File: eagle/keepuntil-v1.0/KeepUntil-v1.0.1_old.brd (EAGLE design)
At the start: 37 x 45 mm, 18 parts, among them IC2 REG1117, J2 USBSMD, Q1 CSTCR6M00G53Z, T1 BC846, U1 ATMEGA328P-AU

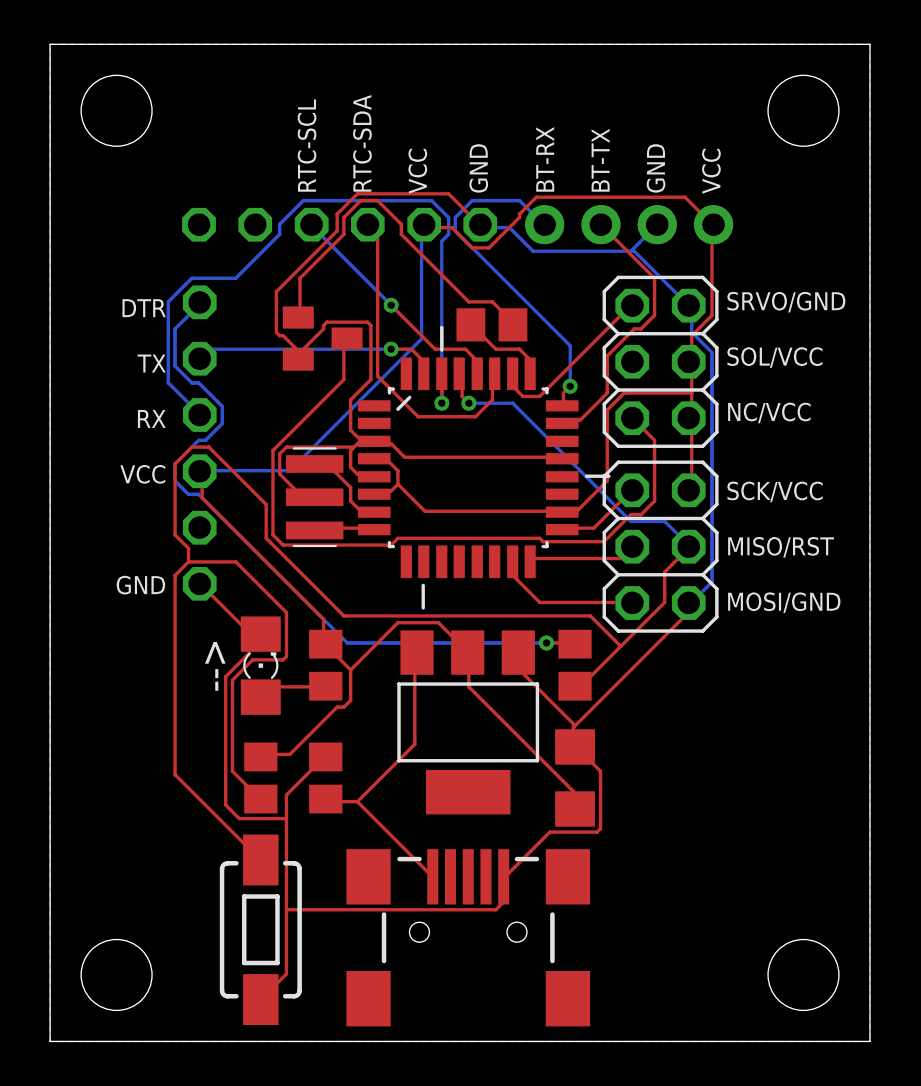
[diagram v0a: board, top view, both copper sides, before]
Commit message: new board layout
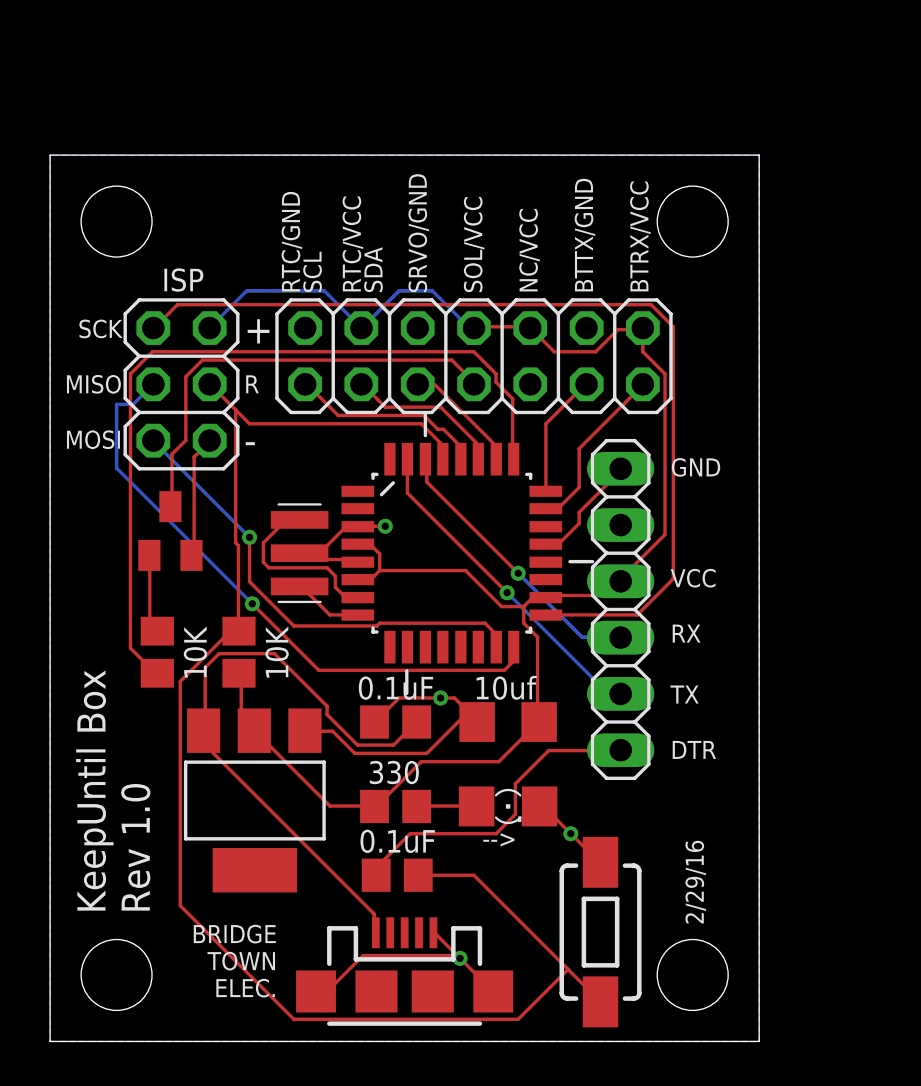
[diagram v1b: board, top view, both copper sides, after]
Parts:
- removed BLUETOOTH: 1X4-CLEANBIG, adafruit:1X04-CLEANBIG
- removed J2: USBSMD, SparkFun-Connectors:USB-MINIB
- removed LOCK-CTRL: (no value), pinhead:2X03
- removed RTC, RTC1: (no value), adafruit:1X06-CLEAN
- added J1: USB-MICROB, SparkFun-Connectors:USB-MICROB
- added JP1: (no value), pinhead:2X07
- added SERIAL: (no value), pinhead:1X06
- C1, C4: value .1uF -> 0.1uF
- moved ISP 22.8 mm to (5.93, 29.7)
- moved R2 21.1 mm to (4.84, 17.6), turned to 270 degrees
- moved S1 15.3 mm to (24.8, 4.93), turned to 270 degrees
- moved LED1 12.8 mm to (20.7, 10.6), turned to 0 degrees
- moved C1 12.4 mm to (15.7, 7.50), turned to 180 degrees
- moved T1 11.1 mm to (5.43, 23.0), turned to 0 degrees
- moved IC2 10.3 mm to (9.24, 10.9)
- moved R7 7.11 mm to (15.6, 10.6), turned to 180 degrees
- moved R1 5.76 mm to (8.53, 17.6), turned to 270 degrees
- moved C4 4.04 mm to (15.6, 14.4), turned to 180 degrees
- moved C2 3.94 mm to (20.7, 14.4), turned to 180 degrees
- moved U1 3.93 mm to (18.1, 22.0)
- moved Q1 2.61 mm to (11.3, 22.0)
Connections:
- net SOL-SIG renamed SOLENOID-SIG
- net BT-RX: now also JP1.2; no longer BLUETOOTH.3
- net BT-TX: now also JP1.4; no longer BLUETOOTH.4
- net GND: now also J1.GND, J1.MT1, J1.MT2, JP1.13, JP1.3, JP1.9, SERIAL.1; no longer BLUETOOTH.2, J2.GND, LOCK-CTRL.2, RTC.1, RTC1.1
- net N$17: now also SERIAL.6; no longer RTC1.6
- net N$4: now also J1.VBUS; no longer J2.VBUS
- net RTC-SCL: now also JP1.14; no longer RTC.4
- net RTC-SDA: now also JP1.12; no longer RTC.3
- net RX: now also SERIAL.4; no longer RTC1.4
- net SERVO: now also JP1.10; no longer LOCK-CTRL.1
- net SOLENOID: now also JP1.8; no longer LOCK-CTRL.5
- net TX: now also SERIAL.5; no longer RTC1.5
- net VCC: now also JP1.1, JP1.11, JP1.5, JP1.7, SERIAL.3; no longer BLUETOOTH.1, LOCK-CTRL.4, LOCK-CTRL.6, RTC.2, RTC1.3
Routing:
- net GND: track 133.1 -> 47.6 mm, vias 0 -> 4
- net SCK: track 3.90 -> 42.1 mm
- net SOLENOID-SIG: track 3.95 -> 35.6 mm
- net VCC: track 100.8 -> 75.3 mm
- net MISO: track 4.91 -> 27.4 mm, vias 0 -> 1
- net RX: track 30.6 -> 12.7 mm
- net N$17: track 31.7 -> 14.4 mm, vias 1 -> 0
- net RESET: track 83.9 -> 67.7 mm, vias 1 -> 0
- net MOSI: track 6.53 -> 21.0 mm, vias 0 -> 1
- net N$4: track 14.2 -> 27.4 mm
- net SOLENOID: track 32.8 -> 20.0 mm
- net N$3: track 16.0 -> 3.56 mm
- net BT-TX: track 15.6 -> 5.61 mm, vias 1 -> 0
- net RTC-SDA: track 14.5 -> 7.04 mm
- net BT-RX: track 12.3 -> 7.79 mm
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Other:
- board size 37 x 45 mm -> 32 x 40 mm
- board text added: "+"
- board text added: "-"
- board text added: "2/29/16"
- board text added: "BRIDGE TOWN ELEC."
- board text added: "BTRX/VCC"
- board text added: "BTTX/GND"
- board text added: "KeepUntil Box"
- board text added: "MISO"
- board text added: "MOSI"
- board text added: "R"
- board text added: "RTC/GND SCL"
- board text added: "RTC/VCC SDA"
- board text added: "Rev 1.0"
- board text added: "SCK"
- board text removed: "BT-RX"
- board text removed: "BT-TX"
- board text removed: "MISO/RST"
- board text removed: "MOSI/GND"
- board text removed: "RTC-SCL"
- board text removed: "RTC-SDA"
- board text removed: "SCK/VCC"
